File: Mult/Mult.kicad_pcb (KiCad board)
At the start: 2 copper layers, 9.7 x 101.3 mm, 5 parts, among them J1 IN, J2 OUT1, J3 OUT2, J4 OUT3, J5 OUT4

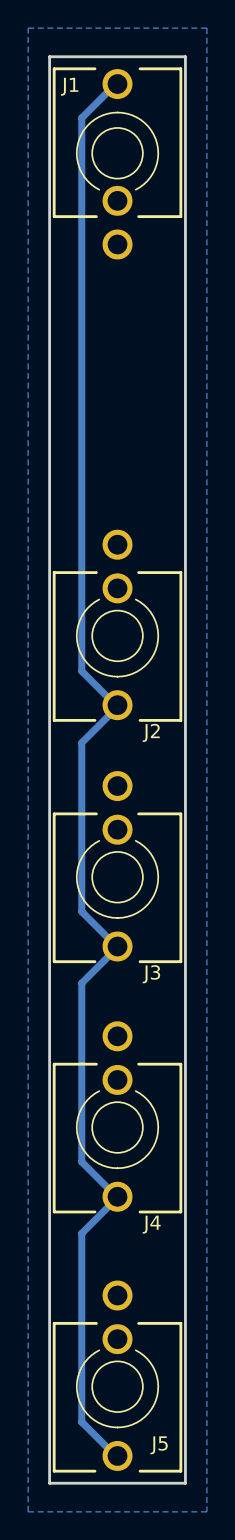
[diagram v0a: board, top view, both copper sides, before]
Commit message: rearrange a bunch of files
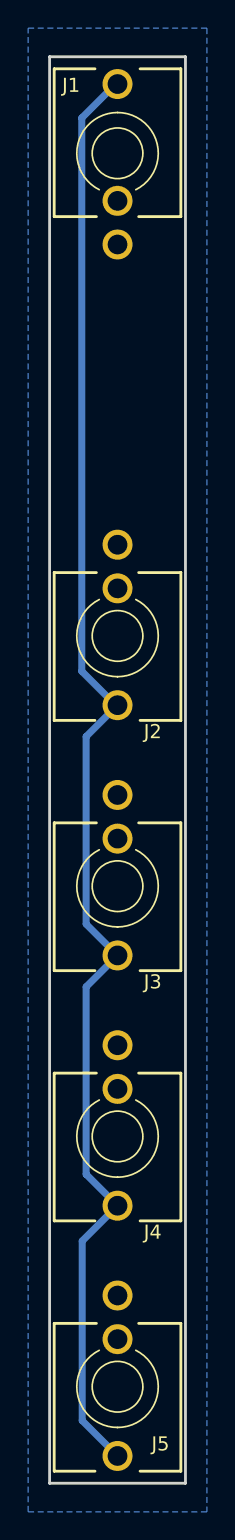
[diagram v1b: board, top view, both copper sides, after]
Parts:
- moved J4 0.64 mm to (152.7, 131.3)
- moved J3 0.63 mm to (152.7, 113.5)
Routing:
- net Net-(J1-PadT): track 106.1 -> 105.6 mm
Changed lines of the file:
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@@
     (grid_origin 147.828 54.58)
     (pcbplotparams
-      (layerselection 0x00010fc_ffffffff)
+      (layerselection 0x0001000_fffffffe)
       (disableapertmacros false)
       (usegerberextensions false)
@@
       (viasonmask false)
       (mode 1)
-      (useauxorigin false)
+      (useauxorigin true)
       (hpglpennumber 1)
       (hpglpenspeed 20)
@@
       (outputformat 1)
       (mirror false)
-      (drillshape 1)
+      (drillshape 0)
       (scaleselection 1)
       (outputdirectory "")
@@
   )
   (footprint "pj398m:Jack_3.5mm_QingPu_WQP-PJ398SM_Vertical" (layer "F.Cu")
-    (at 152.654 112.873 180)
+    (at 152.654 113.508 180)
     (descr "T-S-SN Vertical mount jack AKA WQP-WQP518MA or Thonkiconn")
     (tags "WQP-WQP518MA, Thonkiconn")
@@
   )
   (footprint "pj398m:Jack_3.5mm_QingPu_WQP-PJ398SM_Vertical" (layer "F.Cu")
-    (at 152.654 130.653 180)
+    (at 152.654 131.288 180)
     (descr "T-S-SN Vertical mount jack AKA WQP-WQP518MA or Thonkiconn")
     (tags "WQP-WQP518MA, Thonkiconn")
@@
   (gr_line (start 147.828 155.926) (end 147.828 54.58) (layer "Edge.Cuts") (width 0.2))
   (gr_line (start 157.48 54.58) (end 157.48 155.926) (layer "Edge.Cuts") (width 0.2))
-  (segment (start 150.114 133.098) (end 150.114 120.398) (width 0.5) (layer "B.Cu") (net 2))
-  (segment (start 152.654 117.858) (end 150.114 120.398) (width 0.5) (layer "B.Cu") (net 2))
+  (dimension (type aligned) (layer "User.1")
+    (pts (xy 152.654 61.438) (xy 152.654 54.58))
+    (height -7.366)
+    (gr_text "6.8580 mm" (at 144.138 58.009 90) (layer "User.1")
+      (effects (font (size 1 1) (thickness 0.15)))
+    )
+    (format (units 3) (units_format 1) (precision 4))
+    (style (thickness 0.1) (arrow_length 1.27) (text_position_mode 0) (extension_height 0.58642) (extension_offset 0.5) keep_text_aligned)
+  )
+  (dimension (type aligned) (layer "User.1")
+    (pts (xy 152.654 149.048) (xy 152.654 54.58))
+    (height 10.414)
+    (gr_text "94.4680 mm" (at 161.918 101.814 90) (layer "User.1")
+      (effects (font (size 1 1) (thickness 0.15)))
+    )
+    (format (units 3) (units_format 1) (precision 4))
+    (style (thickness 0.1) (arrow_length 1.27) (text_position_mode 0) (extension_height 0.58642) (extension_offset 0.5) keep_text_aligned)
+  )
+  (dimension (type aligned) (layer "User.1")
+    (pts (xy 152.654 151.098) (xy 147.828 151.1))
+    (height -12.701051)
+    (gr_text "4.8260 mm" (at 150.245787 162.65005 0.02374462339) (layer "User.1")
+      (effects (font (size 1 1) (thickness 0.15)))
+    )
+    (format (units 3) (units_format 1) (precision 4))
+    (style (thickness 0.1) (arrow_length 1.27) (text_position_mode 0) (extension_height 0.58642) (extension_offset 0.5) keep_text_aligned)
+  )
+  (dimension (type orthogonal) (layer "User.1")
+    (pts (xy 152.654 149.068) (xy 152.654 131.288))
+    (height 18.034)
+    (orientation 1)
+    (gr_text "17.7800 mm" (at 169.538 140.178 90) (layer "User.1")
+      (effects (font (size 1 1) (thickness 0.15)))
+    )
+    (format (units 3) (units_format 1) (precision 4))
+    (style (thickness 0.15) (arrow_length 1.27) (text_position_mode 0) (extension_height 0.58642) (extension_offset 0.5) keep_text_aligned)
+  )
+  (segment (start 150.144 138.718) (end 152.654 136.208) (width 0.5) (layer "B.Cu") (net 2))
+  (segment (start 150.423318 120.658682) (end 152.654 118.428) (width 0.5) (layer "B.Cu") (net 2))
   (segment (start 152.654 100.778) (end 150.114 98.238) (width 0.5) (layer "B.Cu") (net 2))
+  (segment (start 150.423318 102.878682) (end 150.423318 116.197318) (width 0.5) (layer "B.Cu") (net 2))
   (segment (start 150.114 98.238) (end 150.114 58.928) (width 0.5) (layer "B.Cu") (net 2))
-  (segment (start 152.654 154.118) (end 150.144 151.608) (width 0.5) (layer "B.Cu") (net 2))
-  (segment (start 152.654 135.638) (end 150.114 138.178) (width 0.5) (layer "B.Cu") (net 2))
-  (segment (start 150.114 115.318) (end 150.114 103.318) (width 0.5) (layer "B.Cu") (net 2))
   (segment (start 150.114 58.928) (end 152.654 56.388) (width 0.5) (layer "B.Cu") (net 2))
-  (segment (start 150.114 103.318) (end 152.654 100.778) (width 0.5) (layer "B.Cu") (net 2))
-  (segment (start 150.144 151.608) (end 150.114 151.608) (width 0.5) (layer "B.Cu") (net 2))
-  (segment (start 152.654 135.638) (end 150.114 133.098) (width 0.5) (layer "B.Cu") (net 2))
-  (segment (start 150.114 138.178) (end 150.114 151.578) (width 0.5) (layer "B.Cu") (net 2))
-  (segment (start 152.654 117.858) (end 150.114 115.318) (width 0.5) (layer "B.Cu") (net 2))
+  (segment (start 152.654 136.208) (end 150.423318 133.977318) (width 0.5) (layer "B.Cu") (net 2))
+  (segment (start 150.423318 133.977318) (end 150.423318 120.658682) (width 0.5) (layer "B.Cu") (net 2))
+  (segment (start 150.423318 116.197318) (end 152.654 118.428) (width 0.5) (layer "B.Cu") (net 2))
+  (segment (start 152.654 100.648) (end 150.423318 102.878682) (width 0.5) (layer "B.Cu") (net 2))
+  (segment (start 150.144 138.718) (end 150.144 151.478) (width 0.5) (layer "B.Cu") (net 2))
+  (segment (start 150.144 151.478) (end 152.654 153.988) (width 0.5) (layer "B.Cu") (net 2))
   (zone (net 1) (net_name "GND") (layer "B.Cu") (hatch edge 0.508)
     (connect_pads (clearance 0.508))
